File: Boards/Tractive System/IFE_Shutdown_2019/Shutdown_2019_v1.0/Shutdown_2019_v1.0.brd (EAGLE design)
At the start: 88.9 x 76.2 mm, 195 parts, among them Q1 DMN6140L-7, Q10 DMN6140L-7, Q11 DMP3099L-7, Q12 IRLML6346PBF, Q13 IRLML6346PBF, Q14 IRLML6346PBF, Q15 DMP3099L-7, Q16 DMN6140L-7, Q17 IRLML6346PBF, Q18 DMN6140L-7, Q2 DMN6140L-7, Q20 DMN6140L-7, Q21 DMN6140L-7, Q3 DMN6140L-7, Q4 DMN6140L-7, Q5 DMN6140L-7, Q6 DMP3099L-7, Q7 DMN6140L-7, Q9 DMN6140L-7, U1 STM32F103CBT6, U2 STM32F103CBT6

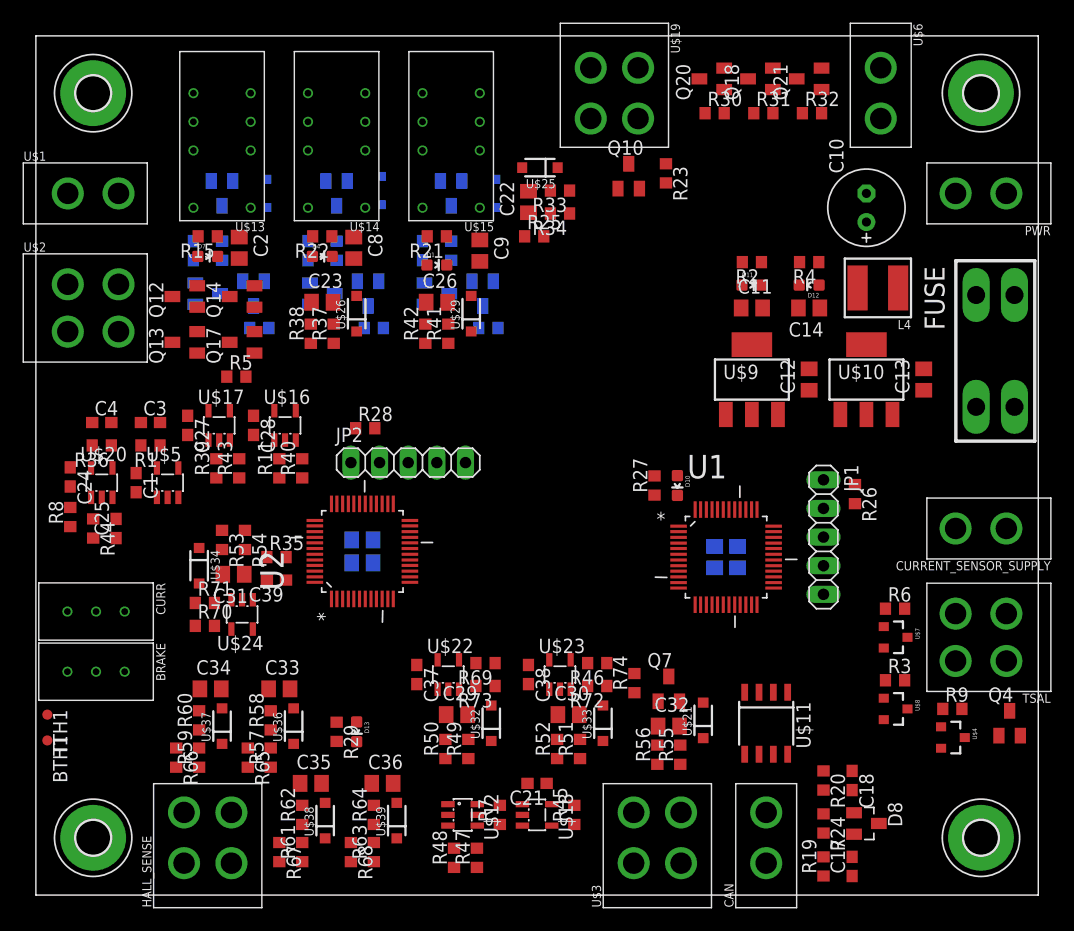
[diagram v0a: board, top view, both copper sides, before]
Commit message: nearly done with routing
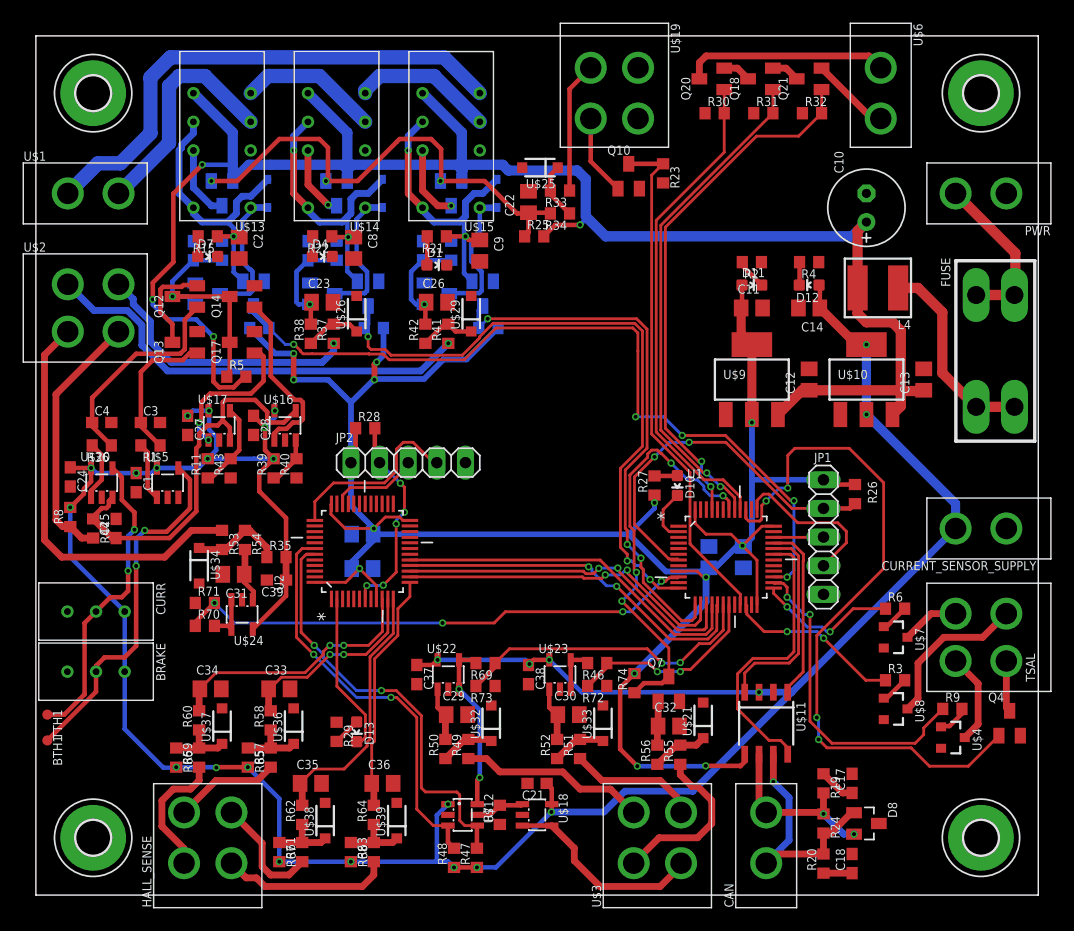
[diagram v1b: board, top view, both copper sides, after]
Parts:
- removed R45: 10k, rcl:R0603
- moved C17 7.37 mm to (72.4, 9.91)
- moved R19 7.37 mm to (69.8, 9.91), turned to 270 degrees
- moved C18 7.37 mm to (72.4, 2.79), turned to 90 degrees
- moved R20 7.37 mm to (69.8, 2.79), turned to 90 degrees
- moved R11 6.35 mm to (15.2, 37.8)
- moved R39 5.08 mm to (21.1, 37.8)
- moved R43 0.76 mm to (17.3, 37.8)
- moved C15 0.51 mm to (59.7, 30.0)
- moved C19 0.51 mm to (62.7, 30.0)
- moved C16 0.51 mm to (29.0, 29.0)
- moved C20 0.51 mm to (29.0, 32.0)
- moved R40 0.51 mm to (23.1, 37.8)
- moved D9 0.25 mm to (30.7, 62.2)
- moved R23 0.25 mm to (55.6, 64.0)
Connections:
- net +5V: no longer R45.2
- net CANH: now also CAN.2; no longer CAN.1
- net CANL: now also CAN.1; no longer CAN.2
- net HALL_FL_F: now also U2.11; no longer U2.25
- net HALL_FR_F: now also U2.10; no longer U2.26
- net HALL_RL_F: now also U2.12; no longer U2.27
- net HALL_RR_F: now also U2.13; no longer U2.28
- net THROTTLE_OUT: no longer R45.1
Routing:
- net +5V: track 0.00 -> 241.0 mm, vias 0 -> 25
- net +3V3: track 0.00 -> 194.4 mm, vias 0 -> 13
- net +12V: track 0.00 -> 161.4 mm, vias 0 -> 4
- net FAULT_BSPD_STATUS_3_3: track 0.00 -> 70.7 mm, vias 0 -> 5
- net RTDS_EN: track 0.00 -> 62.8 mm, vias 0 -> 4
- net FAULT_BMS_STATUS_3_3: track 0.00 -> 57.2 mm, vias 0 -> 3
- net FAULT_IMD_STATUS_3_3: track 0.00 -> 48.9 mm, vias 0 -> 3
- net RTD_EN: track 0.00 -> 47.2 mm, vias 0 -> 2
- net BRAKE_PRESSURE_F_3_3: track 0.00 -> 46.3 mm, vias 0 -> 4
- net HV_CONNECTED_3_3: track 0.00 -> 45.8 mm
- net AIR_OUT: track 0.00 -> 45.8 mm
- net BTSF_EN: track 0.00 -> 44.4 mm, vias 0 -> 2
- net APPS_EN: track 0.00 -> 43.9 mm
- net FAULT_RESET_F: track 0.00 -> 43.5 mm, vias 0 -> 3
- net FAULT_IMD: track 0.00 -> 39.0 mm, vias 0 -> 1
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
